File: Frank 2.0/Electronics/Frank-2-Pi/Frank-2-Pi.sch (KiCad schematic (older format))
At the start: 50 parts, among them J1 left wheel sensor, J10 USB-to-controller, J11 power-connector, J12 servo 3, J13 servo 2, J14 servo 1, J15 GPIO, J16 data-connector, J2 Left motor, J3 Right motor, J4 right wheel sensor, J5 Analogue inputs, J6 LIDAR, J7 Phototransistor, J8 USB-from-battery, J9 power switch, Q1 DMN6075S, Q2 DMN6075S, U1 adafruit-2448, U2 LM2903, U3 adafruit-1015, U4 AP1117-33, U5 sparkfun-sx1509

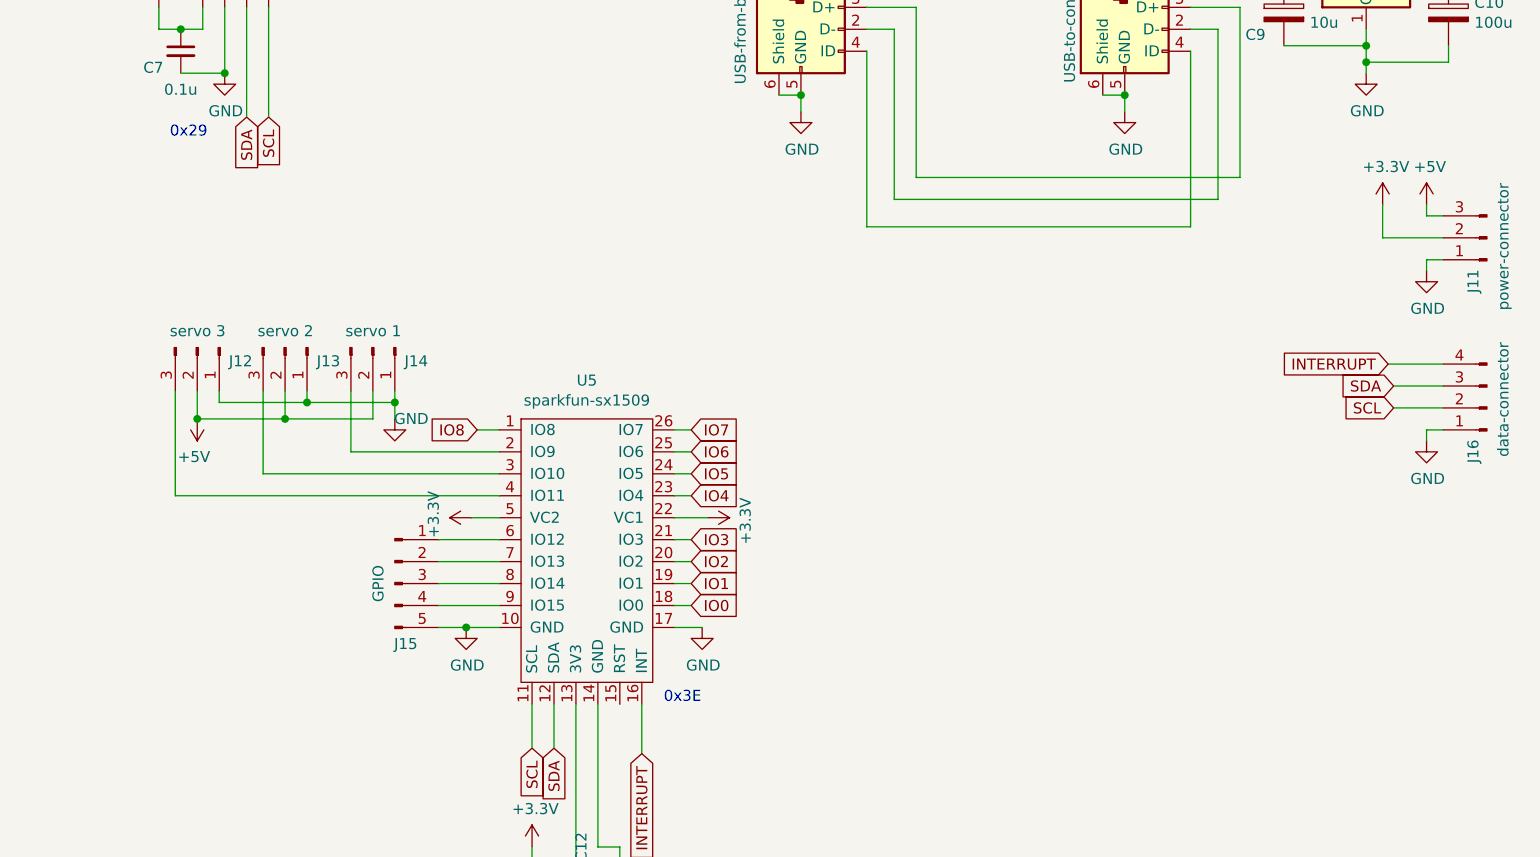
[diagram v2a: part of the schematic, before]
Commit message: Now with indicator LEDs...
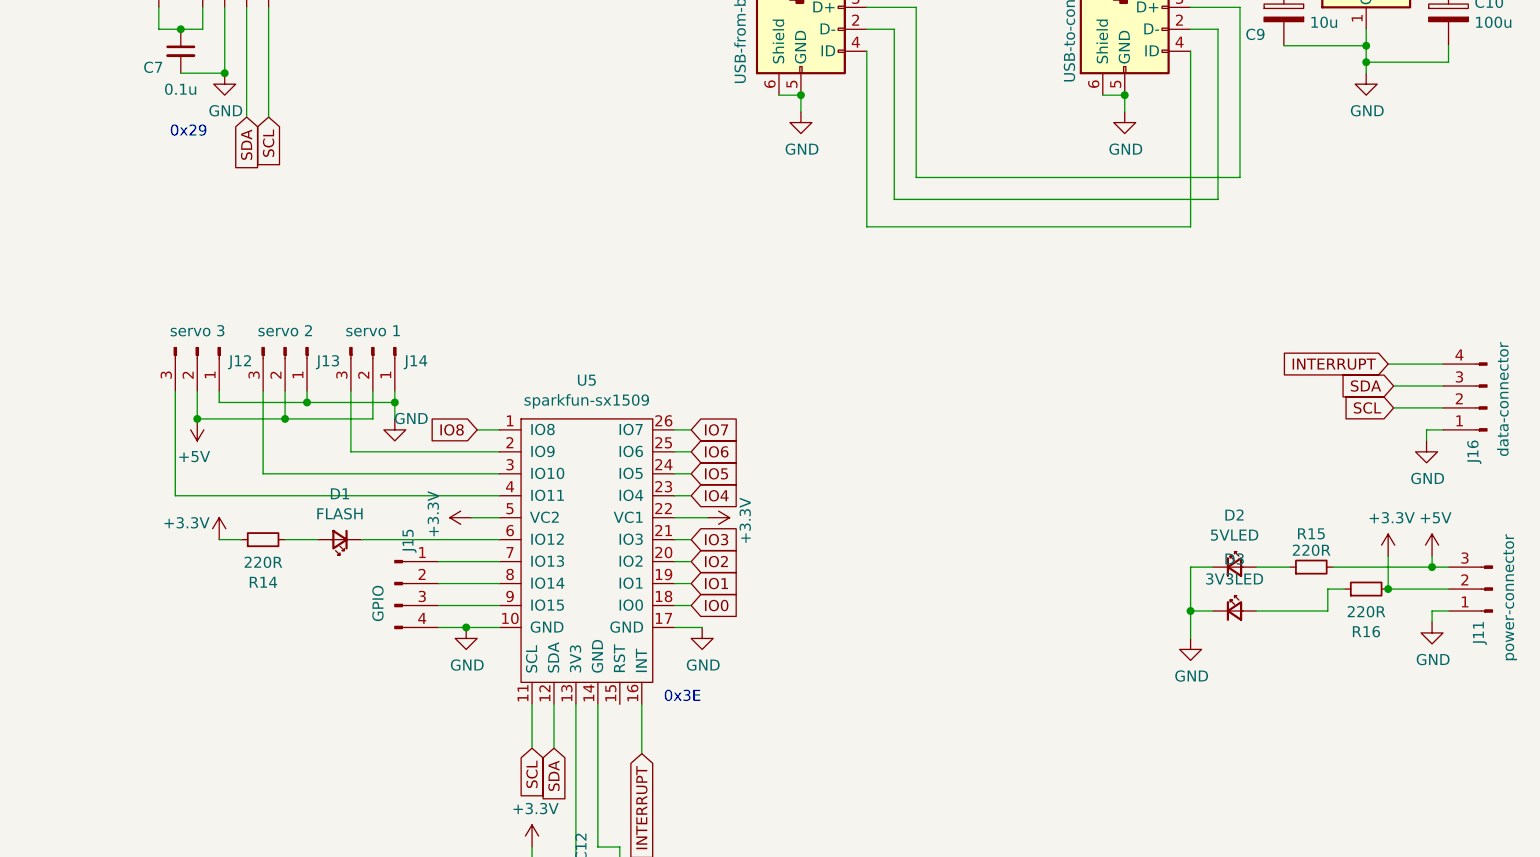
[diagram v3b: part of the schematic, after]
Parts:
- removed J15: GPIO, Connector_PinHeader_2.54mm:PinHeader_1x05_P2.54mm_Vertical, symbol Connector:Conn_01x05_Male
- added D1: FLASH, LED_SMD:LED_0805_2012Metric, symbol Device:LED_Small
- added D2: 5VLED, LED_SMD:LED_0805_2012Metric, symbol Device:LED_Small
- added D3: 3V3LED, LED_SMD:LED_0805_2012Metric, symbol Device:LED_Small
- added J15: GPIO, Connector_PinHeader_2.54mm:PinHeader_1x04_P2.54mm_Vertical, symbol Connector:Conn_01x04_Male
- added R14, R15, R16: 220R, Resistor_SMD:R_0805_2012Metric, symbol Device:R_Small
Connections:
- net +3V3: now also R14.1, R16.2
- net +5V: now also R15.2
- net GND: now also D2.1 (K), D3.1 (K), J15.4 (Pin_4)
- net at U5.6 (IO12): now also D1.1 (K)
- net at U5.7 (IO13): now also J15.1 (Pin_1)
- net at U5.8 (IO14): now also J15.2 (Pin_2)
- net at U5.9 (IO15): now also J15.3 (Pin_3)
- new net: D3.2 (A), R16.1
- new net: D2.2 (A), R15.1
- new net: D1.2 (A), R14.2
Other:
- moved on the sheet: J11
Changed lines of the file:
@@
 L Connector:Conn_01x03_Male J11
 U 1 1 5F0CD551
-P 10925 2100
-F 0 "J11" V 10987 2244 50  0000 L CNN
-F 1 "power-connector" V 10850 1850 50  0000 L CNN
-F 2 "Connector_PinHeader_2.54mm:PinHeader_1x03_P2.54mm_Vertical" H 10925 2100 50  0001 C CNN
-F 3 "~" H 10925 2100 50  0001 C CNN
-	1    10925 2100
+P 10950 3700
+F 0 "J11" V 11012 3844 50  0000 L CNN
+F 1 "power-connector" V 10875 3450 50  0000 L CNN
+F 2 "Connector_PinHeader_2.54mm:PinHeader_1x03_P2.54mm_Vertical" H 10950 3700 50  0001 C CNN
+F 3 "~" H 10950 3700 50  0001 C CNN
+	1    10950 3700
 	-1   0    0    1
 $EndComp
@@
 L power:+5V #PWR0135
 U 1 1 5F0CF071
-P 10650 1950
-F 0 "#PWR0135" H 10650 1800 50  0001 C CNN
-F 1 "+5V" H 10665 2123 50  0000 C CNN
-F 2 "" H 10650 1950 50  0001 C CNN
-F 3 "" H 10650 1950 50  0001 C CNN
-	1    10650 1950
+P 10675 3550
+F 0 "#PWR0135" H 10675 3400 50  0001 C CNN
+F 1 "+5V" H 10690 3723 50  0000 C CNN
+F 2 "" H 10675 3550 50  0001 C CNN
+F 3 "" H 10675 3550 50  0001 C CNN
+	1    10675 3550
 	1    0    0    -1
 $EndComp
@@
 L power:+3.3V #PWR0136
 U 1 1 5F0CF608
-P 10450 1950
-F 0 "#PWR0136" H 10450 1800 50  0001 C CNN
-F 1 "+3.3V" H 10465 2123 50  0000 C CNN
-F 2 "" H 10450 1950 50  0001 C CNN
-F 3 "" H 10450 1950 50  0001 C CNN
-	1    10450 1950
+P 10475 3550
+F 0 "#PWR0136" H 10475 3400 50  0001 C CNN
+F 1 "+3.3V" H 10490 3723 50  0000 C CNN
+F 2 "" H 10475 3550 50  0001 C CNN
+F 3 "" H 10475 3550 50  0001 C CNN
+	1    10475 3550
 	1    0    0    -1
 $EndComp
@@
 L power:GND #PWR0137
 U 1 1 5F0CFC12
-P 10650 2250
-F 0 "#PWR0137" H 10650 2000 50  0001 C CNN
-F 1 "GND" H 10655 2077 50  0000 C CNN
-F 2 "" H 10650 2250 50  0001 C CNN
-F 3 "" H 10650 2250 50  0001 C CNN
-	1    10650 2250
-	1    0    0    -1
-$EndComp
-Wire Wire Line
-	10725 2200 10650 2200
-Wire Wire Line
-	10650 2200 10650 2250
-Wire Wire Line
-	10725 2100 10450 2100
-Wire Wire Line
-	10450 2100 10450 1950
-Wire Wire Line
-	10725 2000 10650 2000
-Wire Wire Line
-	10650 2000 10650 1950
+P 10675 3850
+F 0 "#PWR0137" H 10675 3600 50  0001 C CNN
+F 1 "GND" H 10680 3677 50  0000 C CNN
+F 2 "" H 10675 3850 50  0001 C CNN
+F 3 "" H 10675 3850 50  0001 C CNN
+	1    10675 3850
+	1    0    0    -1
+$EndComp
+Wire Wire Line
+	10750 3800 10675 3800
+Wire Wire Line
+	10675 3800 10675 3850
+Wire Wire Line
+	10750 3700 10475 3700
+Wire Wire Line
+	10750 3600 10675 3600
+Wire Wire Line
+	10675 3600 10675 3550
 $Comp
 L power:GND #PWR0138
@@
 	5850 2925 5850 2800
 Connection ~ 5450 2925
-$Comp
-L Connector:Conn_01x05_Male J15
-U 1 1 5F116CDD
-P 5950 3675
-F 0 "J15" H 6000 3400 50  0000 C CNN
-F 1 "GPIO" V 5875 3675 50  0000 C CNN
-F 2 "Connector_PinHeader_2.54mm:PinHeader_1x05_P2.54mm_Vertical" H 5950 3675 50  0001 C CNN
-F 3 "~" H 5950 3675 50  0001 C CNN
-	1    5950 3675
-	1    0    0    -1
-$EndComp
-Wire Wire Line
-	6150 3475 6425 3475
 Wire Wire Line
 	6150 3575 6425 3575
@@
 	6575 5000 6575 4875
 Connection ~ 6775 5000
+$Comp
+L Device:R_Small R16
+U 1 1 5EC9242B
+P 10375 3700
+F 0 "R16" V 10179 3700 50  0000 C CNN
+F 1 "220R" V 10270 3700 50  0000 C CNN
+F 2 "Resistor_SMD:R_0805_2012Metric" H 10375 3700 50  0001 C CNN
+F 3 "~" H 10375 3700 50  0001 C CNN
+	1    10375 3700
+	0    -1   -1   0
+$EndComp
+$Comp
+L Device:R_Small R15
+U 1 1 5EC93474
+P 10125 3600
+F 0 "R15" V 10275 3600 50  0000 C CNN
+F 1 "220R" V 10200 3600 50  0000 C CNN
+F 2 "Resistor_SMD:R_0805_2012Metric" H 10125 3600 50  0001 C CNN
+F 3 "~" H 10125 3600 50  0001 C CNN
+	1    10125 3600
+	0    -1   -1   0
+$EndComp
+Connection ~ 10475 3700
+Wire Wire Line
+	10475 3550 10475 3700
+Wire Wire Line
+	10675 3600 10225 3600
+Connection ~ 10675 3600
+Wire Wire Line
+	10025 3600 9875 3600
+Wire Wire Line
+	10275 3700 10200 3700
+Wire Wire Line
+	10200 3700 10200 3800
+Wire Wire Line
+	10200 3800 9875 3800
+$Comp
+L power:GND #PWR0145
+U 1 1 5ED22480
+P 9575 3925
+F 0 "#PWR0145" H 9575 3675 50  0001 C CNN
+F 1 "GND" H 9580 3752 50  0000 C CNN
+F 2 "" H 9575 3925 50  0001 C CNN
+F 3 "" H 9575 3925 50  0001 C CNN
+	1    9575 3925
+	1    0    0    -1
+$EndComp
+$Comp
+L Connector:Conn_01x04_Male J15
+U 1 1 5ED486D7
+P 5950 3675
+F 0 "J15" V 6012 3819 50  0000 L CNN
+F 1 "GPIO" V 5875 3500 50  0000 L CNN
+F 2 "Connector_PinHeader_2.54mm:PinHeader_1x04_P2.54mm_Vertical" H 5950 3675 50  0001 C CNN
+F 3 "~" H 5950 3675 50  0001 C CNN
+	1    5950 3675
+	1    0    0    -1
+$EndComp
+$Comp
+L Device:R_Small R14
+U 1 1 5ED6E2BB
+P 5350 3475
+F 0 "R14" V 5154 3475 50  0000 C CNN
+F 1 "220R" V 5245 3475 50  0000 C CNN
+F 2 "Resistor_SMD:R_0805_2012Metric" H 5350 3475 50  0001 C CNN
+F 3 "~" H 5350 3475 50  0001 C CNN
+	1    5350 3475
+	0    -1   -1   0
+$EndComp
+$Comp
+L power:+3.3V #PWR0146
+U 1 1 5ED82DCA
+P 5150 3475
+F 0 "#PWR0146" H 5150 3325 50  0001 C CNN
+F 1 "+3.3V" H 5000 3550 50  0000 C CNN
+F 2 "" H 5150 3475 50  0001 C CNN
+F 3 "" H 5150 3475 50  0001 C CNN
+	1    5150 3475
+	1    0    0    -1
+$EndComp
+Wire Wire Line
+	5250 3475 5150 3475
+$Comp
+L Device:LED_Small D1
+U 1 1 5EDA984E
+P 5700 3475
+F 0 "D1" H 5700 3268 50  0000 C CNN
+F 1 "FLASH" H 5700 3359 50  0000 C CNN
+F 2 "LED_SMD:LED_0805_2012Metric" V 5700 3475 50  0001 C CNN
+F 3 "~" V 5700 3475 50  0001 C CNN
+	1    5700 3475
+	-1   0    0    1
+$EndComp
+Wire Wire Line
+	5800 3475 6425 3475
+Wire Wire Line
+	5450 3475 5600 3475
+$Comp
+L Device:LED_Small D2
+U 1 1 5EDD6E16
+P 9775 3600
+F 0 "D2" H 9775 3835 50  0000 C CNN
+F 1 "5VLED" H 9775 3744 50  0000 C CNN
+F 2 "LED_SMD:LED_0805_2012Metric" V 9775 3600 50  0001 C CNN
+F 3 "~" V 9775 3600 50  0001 C CNN
+	1    9775 3600
+	1    0    0    -1
+$EndComp
+Wire Wire Line
+	9575 3600 9575 3800
+$Comp
+L Device:LED_Small D3
+U 1 1 5EDDE768
+P 9775 3800
+F 0 "D3" H 9775 4035 50  0000 C CNN
+F 1 "3V3LED" H 9775 3944 50  0000 C CNN
+F 2 "LED_SMD:LED_0805_2012Metric" V 9775 3800 50  0001 C CNN
+F 3 "~" V 9775 3800 50  0001 C CNN
+	1    9775 3800
+	1    0    0    -1
+$EndComp
+Wire Wire Line
+	9675 3600 9575 3600
+Wire Wire Line
+	9675 3800 9575 3800
+Connection ~ 9575 3800
+Wire Wire Line
+	9575 3800 9575 3925
 $EndSCHEMATC
